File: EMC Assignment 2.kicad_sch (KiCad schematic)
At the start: 34 parts, among them IC1 LP2985AIM5-3.0_NOPB, U1 OPA4350, U2 OPA4350, U3 OPA4350, U4 OPA4350

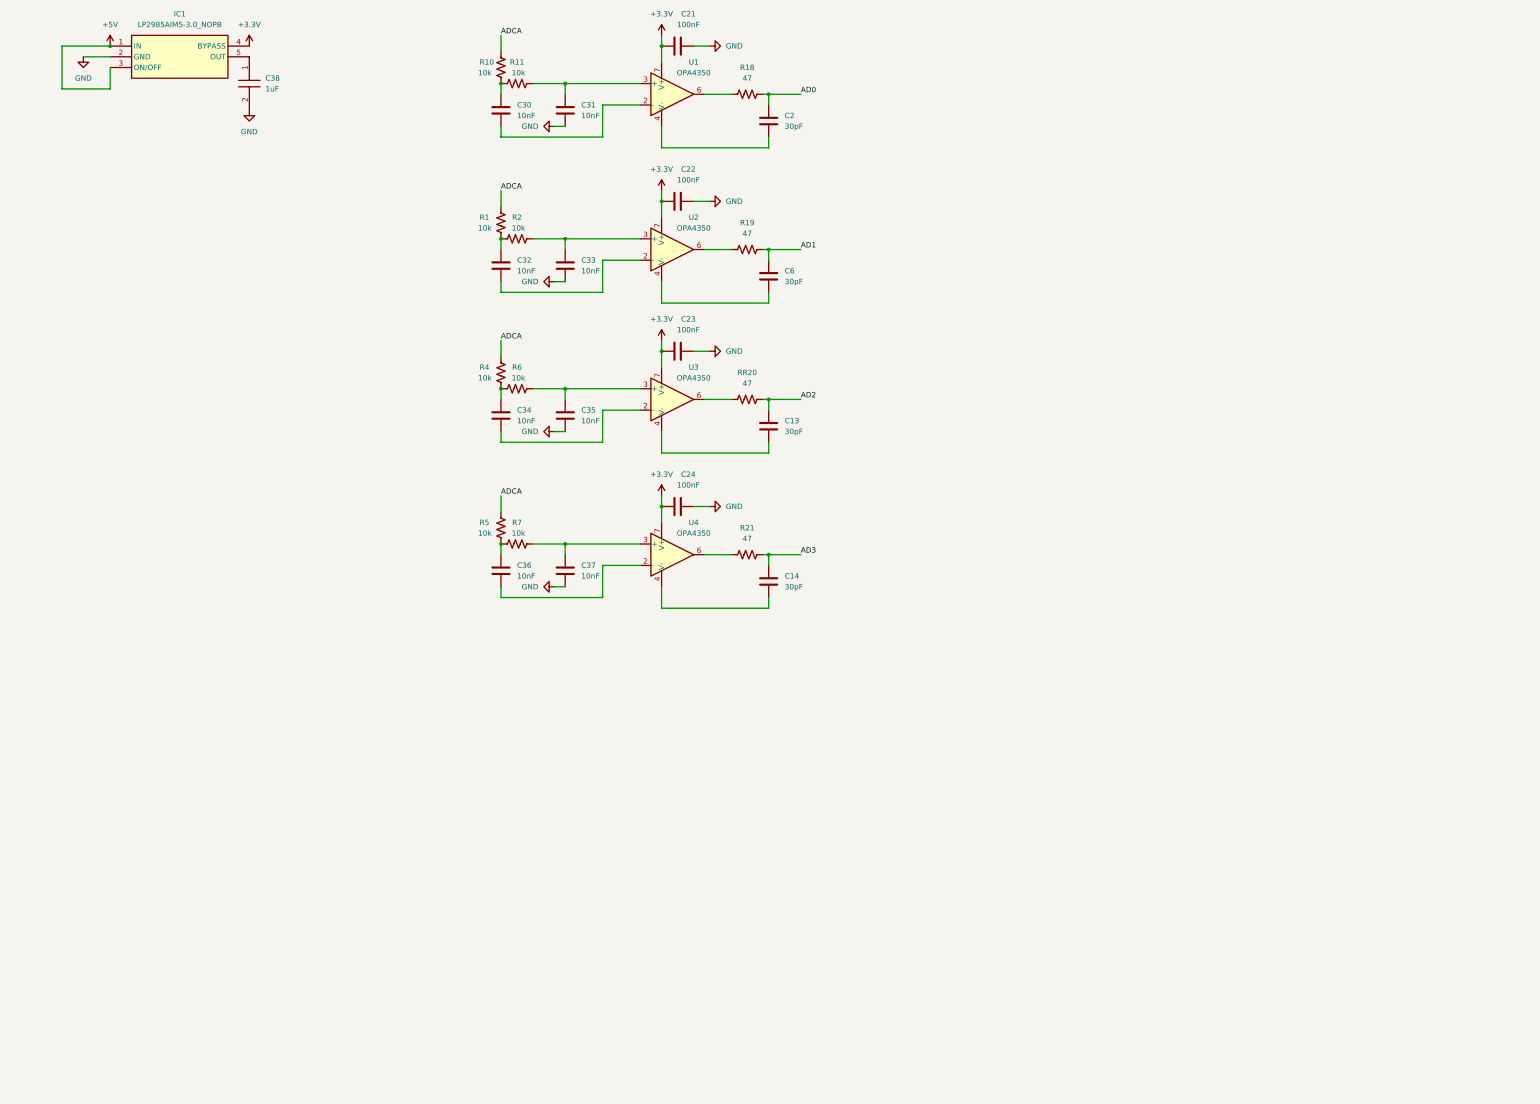
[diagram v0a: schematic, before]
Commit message: Pushed the right build this time o.0
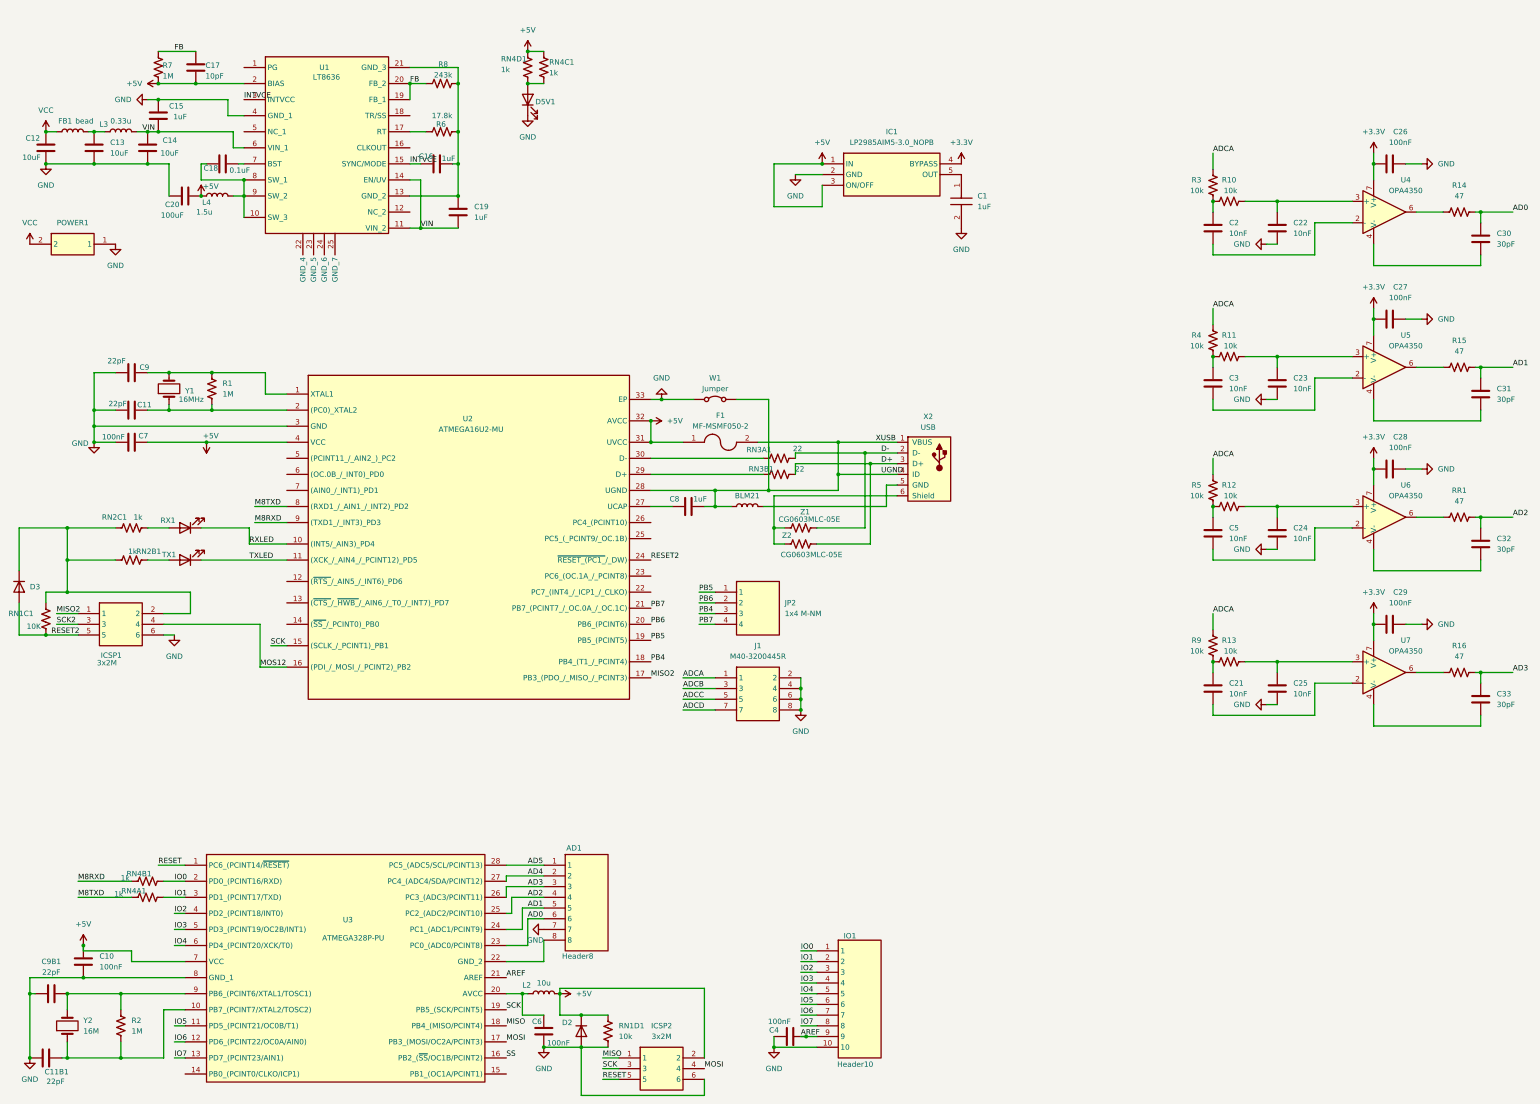
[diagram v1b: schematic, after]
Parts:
- removed C34, C35, C36, C37: 10nF, symbol Device:C
- removed C38: 1uF, CAPC2012X140N, symbol 0805ZC105KAZ2A:0805ZC105KAZ2A
- removed R18, R19, R21, RR20: 47, symbol Device:R_US
- removed U1, U2, U3: OPA4350, symbol Amplifier_Operational:OPA1641
- added AD1: Header8, HDRV8W69P0X254_1X8_2032X251X1641P, symbol 87891-0808:87891-0808
- added BLM21: L, BLM21:BLM21AG102BH1J, symbol Device:L
- added C1: 1uF, Capacitor_SMD:C_0805_2012Metric, symbol 0805ZC105KAZ2A:0805ZC105KAZ2A
- added C10, C4, C7: 100nF, C0805C112F5GACTU//:C0805, symbol Device:C
- added C11, C11B1, C9, C9B1: 22pF, C0805C112F5GACTU//:C0805, symbol Device:C
- added C12: 10uF, C0805C112F5GACTU//:C0805, symbol Device:C
- added C15, C16, C19, C8: 1uF, C0805C112F5GACTU//:C0805, symbol Device:C
- added C17: 10pF, C0805C112F5GACTU//:C0805, symbol Device:C
- added C18: 0.1uF, C0805C112F5GACTU//:C0805, symbol Device:C
- added C20: 100uF, C0805C112F5GACTU//:C0805, symbol Device:C
- added C25, C3: 10nF, Capacitor_SMD:C_0805_2012Metric, symbol Device:C
- added C26, C27, C29: 100nF, Capacitor_SMD:C_0805_2012Metric, symbol Device:C
- added C28: 100nF, symbol Device:C
- added C5: 10nF, symbol Device:C
- added D2: 1N4148WT, Diode_SMD:D_SOD-523, symbol Diode:1N4148WT
- added D3: D, Diode_SMD:D_0805_2012Metric, symbol Device:D
- added D5V1, RX1, TX1: LED, LED_SMD:LED_0805_2012Metric, symbol Device:LED
- added F1: MF-MSMF050-2, FUSC4632X85N, symbol MF-MSMF050-2:MF-MSMF050-2
- added FB1: bead, Inductor_SMD:L_0805_2012Metric, symbol Device:L
- added ICSP1, ICSP2: 3x2M, M225320305R, symbol M22-5320305R:M22-5320305R
- added IO1: Header10, SHDR10W64P0X250_1X10_2740X575X700P, symbol B10B-XASK-1_LF__SN_:B10B-XASK-1_LF__SN_
- added J1: M40-3200445R, HUSSP8W30P100_2X4_400X320X365P, symbol M40-3200445R:M40-3200445R
- added JP2: 1x4 M-NM, RHDR4W70P0X254_1X4_1056X250X865P, symbol M20-7820446:M20-7820446
- added L2: 10u, Inductor_SMD:L_0805_2012Metric, symbol Device:L
- added L3: 0.33u, Inductor_SMD:L_0805_2012Metric, symbol Device:L
- added L4: 1.5u, Inductor_SMD:L_0805_2012Metric, symbol Device:L
- added POWER1: 3-647166-2, 3-647166-2//, symbol 3-647166-2:3-647166-2
- added R12, R13, R3, R9, RN1D1: 10k, Resistor_SMD:R_0805_2012Metric, symbol Device:R_US
- added R14, R15, R16, RR1: 47, Resistor_SMD:R_0805_2012Metric, symbol Device:R_US
- added R8: 243k, Resistor_SMD:R_0805_2012Metric, symbol Device:R_US
- added RN1C1: 10K, Resistor_SMD:R_0805_2012Metric, symbol Device:R_US
- added RN2B1, RN2C1, RN4A1, RN4B1, RN4C1, RN4D1: 1k, Resistor_SMD:R_0805_2012Metric, symbol Device:R_US
- added RN3A1, RN3B1: 22, Resistor_SMD:R_0805_2012Metric, symbol Device:R_US
- added U1: LT8636, LT8636HVPBF, symbol LT8636HV#PBF:LT8636HV#PBF
- added U2: ATMEGA16U2-MU, QFN50P500X500X100-33N-D, symbol ATMEGA16U2-MU:ATMEGA16U2-MU
- added U3: ATMEGA328P-PU, DIP794W53P254L3467H457Q28N, symbol ATMEGA328P-PU:ATMEGA328P-PU
- added U5, U6, U7: OPA4350, Package_SO:SOIC-8_3.9x4.9mm_P1.27mm, symbol Amplifier_Operational:OPA1641
- added W1: Jumper, Jumper:SolderJumper-2_P1.3mm_Bridged2Bar_Pad1.0x1.5mm, symbol Jumper:Jumper_2_Bridged
- added X2: USB, Connector_USB:USB_Micro-B_Wuerth_614105150721_Vertical, symbol Connector:USB_B_Mini
- added Y1: 16MHz, Crystal:Crystal_SMD_FOX_FE-2Pin_7.5x5.0mm, symbol Device:Crystal
- added Y2: 16M, Crystal:Crystal_SMD_FOX_FE-2Pin_7.5x5.0mm, symbol Device:Crystal
- added Z1, Z2: CG0603MLC-05E, CG0603MLC-05E:VARC1608X55N, symbol Device:R_US
- C13, C14: value 30pF -> 10uF; footprint (none) -> C0805C112F5GACTU//:C0805
- C2: value 30pF -> 10nF; footprint (none) -> Capacitor_SMD:C_0805_2012Metric
- C21, C22, C23: value 100nF -> 10nF; footprint (none) -> Capacitor_SMD:C_0805_2012Metric
- C24: value 100nF -> 10nF
- C30, C31, C32, C33: value 10nF -> 30pF; footprint (none) -> Capacitor_SMD:C_0805_2012Metric
- C6: value 30pF -> 100nF; footprint (none) -> C0805C112F5GACTU//:C0805
- R1, R2, R7: value 10k -> 1M; footprint (none) -> Resistor_SMD:R_0805_2012Metric
- R10, R11, R4, R5: footprint (none) -> Resistor_SMD:R_0805_2012Metric
- R6: value 10k -> 17.8k; footprint (none) -> Resistor_SMD:R_0805_2012Metric
- U4: footprint (none) -> Package_SO:SOIC-8_3.9x4.9mm_P1.27mm
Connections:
- net +3.3V: now also C26.1, C27.1, C28.1, C29.1, U5.7 (V+), U6.7 (V+), U7.7 (V+); no longer C21.1, C22.1, C23.1, C24.1
- net +5V: now also R7.2, C10.1, C17.2, C20.2, C7.2, D2.1 (K), F1.1, ICSP2.2, L2.2, L4.1, RN1D1.1, RN4C1.1, RN4D1.1, U1.2 (BIAS), U2.31 (UVCC), U2.32 (AVCC), U2.4 (VCC), U3.7 (VCC)
- net AD0: now also C30.1, AD1.6, R14.2, U3.23 (PC0_(ADC0/PCINT8)); no longer C2.1
- net AD1: now also C31.1, AD1.5, R15.2, U3.24 (PC1_(ADC1/PCINT9)); no longer C6.1
- net AD2: now also C32.1, AD1.4, RR1.2, U3.25 (PC2_(ADC2/PCINT10)); no longer C13.1
- net AD3: now also C33.1, AD1.3, R16.2, U3.26 (PC3_(ADC3/PCINT11)); no longer C14.1
- net ADCA: now also J1.1, R3.2, R9.2; no longer R1.2, R10.2
- net GND: now also C13.2, C14.2, C6.2, AD1.7, C1.2, C10.2, C11.1, C11B1.1, C12.2, C15.1, C20.1, C25.2, C26.2, C27.2, C28.2, C29.2, C4.1, C7.1, C9.1, C9B1.1, D2.2 (A), D5V1.1 (K), ICSP1.6, ICSP2.6, IO1.10, J1.2, J1.4, J1.6, J1.8, POWER1.1, RN1D1.2, U1.4 (GND_1), U2.3 (GND), U2.33 (EP), U3.8 (GND_1), W1.1 (A); no longer C21.2, C31.2, C33.2
- net at C30.2: now also U4.4 (V-)
- net at R4.1: now also R11.1, C3.1; no longer R6.1
- net at R2.2: now also C11B1.2, U3.10 (PB7_(PCINT7/XTAL2/TOSC2)), Y2.1; no longer C33.1
- net at R11.2: now also C23.1, U5.3 (+); no longer C31.1
- net at R6.2: now also C16.2, C19.1, R8.2, U1.13 (GND_2), U1.21 (GND_3)
- net at U4.6: now also R14.1
- net at C32.2: now also U6.4 (V-)
- net at R5.1: now also C5.1, R12.1; no longer R7.1
- net at U4.3 (+): now also C22.1, R10.2; no longer R7.2
- net at U4.2 (-): now also C2.2
- net at IC1.5 (OUT): now also C1.1
- new net: C9.2, R1.1, U2.1 (XTAL1), Y1.2
- new net: C11.2, R1.2, U2.2 ((PC0)_XTAL2), Y1.1
- new net: C8.1, U2.27 (UCAP)
- new net: RN3B1.1, U2.29 (D+)
- new net: RN3A1.1, U2.30 (D-)
- new net: C25.1, R13.2, U7.3 (+)
- new net: D3.1 (K), ICSP1.2, RN1C1.1, RN2B1.1, RN2C1.1
- new net: C21.2, U7.2 (-)
- new net: C33.2, U7.4 (V-)
- new net: R16.1, U7.6
- new net: C13.1, FB1.2, L3.1
- new net: D5V1.2 (A), RN4C1.2, RN4D1.2
- new net: RR1.1, U6.6
- new net: RN2B1.2, TX1.2 (A)
- new net: C6.1, L2.1, U3.20 (AVCC)
- new net: C9B1.2, R2.1, U3.9 (PB6_(PCINT6/XTAL1/TOSC1)), Y2.2
- new net: C21.1, R13.1, R9.1
- new net: X2.6 (Shield), Z1.1, Z2.1
- new net: BLM21.2, X2.5 (GND)
- new net: C18.1, L4.2, U1.10 (SW_3), U1.8 (SW_1), U1.9 (SW_2)
- new net: R6.1, U1.17 (RT)
- new net: C18.2, U1.7 (BST)
- new net: C3.2, U5.2 (-)
- new net: AD1.8, U3.22 (GND_2)
- new net: C5.2, U6.2 (-)
- new net: C24.1, R12.2, U6.3 (+)
- new net: C2.1, R10.1, R3.1
- new net: C31.2, U5.4 (V-)
- new net: R15.1, U5.6
- new net: RN2C1.2, RX1.2 (A)
- new net AD4: AD1.2, U3.27 (PC4_(ADC4/SDA/PCINT12))
- new net AD5: AD1.1, U3.28 (PC5_(ADC5/SCL/PCINT13))
- new net ADCB: J1.3
- new net ADCC: J1.5
- new net ADCD: J1.7
- new net AREF: C4.2, IO1.9, U3.21 (AREF)
- new net D+: RN3B1.2, X2.3 (D+), Z2.2
- new net D-: RN3A1.2, X2.2 (D-), Z1.2
- new net FB: C17.1, R7.1, R8.1, U1.19 (FB_1), U1.20 (FB_2)
- new net INTVCE: C16.1, U1.15 (SYNC/MODE), U1.3 (INTVCC)
- new net IO0: IO1.1, RN4B1.2, U3.2 (PD0_(PCINT16/RXD))
- new net IO1: IO1.2, RN4A1.2, U3.3 (PD1_(PCINT17/TXD))
- new net IO2: IO1.3, U3.4 (PD2_(PCINT18/INT0))
- new net IO3: IO1.4, U3.5 (PD3_(PCINT19/OC2B/INT1))
- new net IO4: IO1.5, U3.6 (PD4_(PCINT20/XCK/T0))
- new net IO5: IO1.6, U3.11 (PD5_(PCINT21/OC0B/T1))
- new net IO6: IO1.7, U3.12 (PD6_(PCINT22/OC0A/AIN0))
- new net IO7: IO1.8, U3.13 (PD7_(PCINT23/AIN1))
- new net M8RXD: RN4B1.1, U2.9 ((TXD1_/_INT3)_PD3)
- new net M8TXD: RN4A1.1, U2.8 ((RXD1_/_AIN1_/_INT2)_PD2)
- new net MISO: ICSP2.1, U3.18 (PB4_(MISO/PCINT4))
- new net MISO2: ICSP1.1, U2.17 (PB3_(PDO_/_MISO_/_PCINT3))
- new net MOS12: ICSP1.4, U2.16 ((PDI_/_MOSI_/_PCINT2)_PB2)
- new net MOSI: ICSP2.4, U3.17 (PB3_(MOSI/OC2A/PCINT3))
- new net PB4: JP2.3, U2.18 (PB4_(T1_/_PCINT4))
- new net PB5: JP2.1, U2.19 (PB5_(PCINT5))
- new net PB6: JP2.2, U2.20 (PB6_(PCINT6))
- new net PB7: JP2.4, U2.21 (PB7_(PCINT7_/_OC.0A_/_OC.1C))
- new net RESET: ICSP2.5, U3.1 (PC6_(PCINT14/~{RESET)})
- new net RESET2: D3.2 (A), ICSP1.5, RN1C1.2, U2.24 (~{RESET_(PC1_}/_DW))
- new net RXLED: RX1.1 (K), U2.10 ((INT5/_AIN3)_PD4)
- new net SCK: ICSP2.3, U2.15 ((SCLK_/_PCINT1)_PB1), U3.19 (PB5_(SCK/PCINT5))
- new net SCK2: ICSP1.3
- new net SS: U3.16 (PB2_(~{SS}/OC1B/PCINT2))
- new net TXLED: TX1.1 (K), U2.11 ((XCK_/_AIN4_/_PCINT12)_PD5)
- new net UGND: BLM21.1, C8.2, F1.2, U2.28 (UGND), W1.2 (B), X2.1 (VBUS), X2.4 (ID)
- new net VCC: C12.1, FB1.1, POWER1.2
- new net VIN: C14.1, C15.2, C19.2, L3.2, U1.11 (VIN_2), U1.14 (EN/UV), U1.6 (VIN_1)
